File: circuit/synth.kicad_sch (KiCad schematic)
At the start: 3 parts, among them J1 Raspberry_Pi_4, U1 ADS1115IDGS

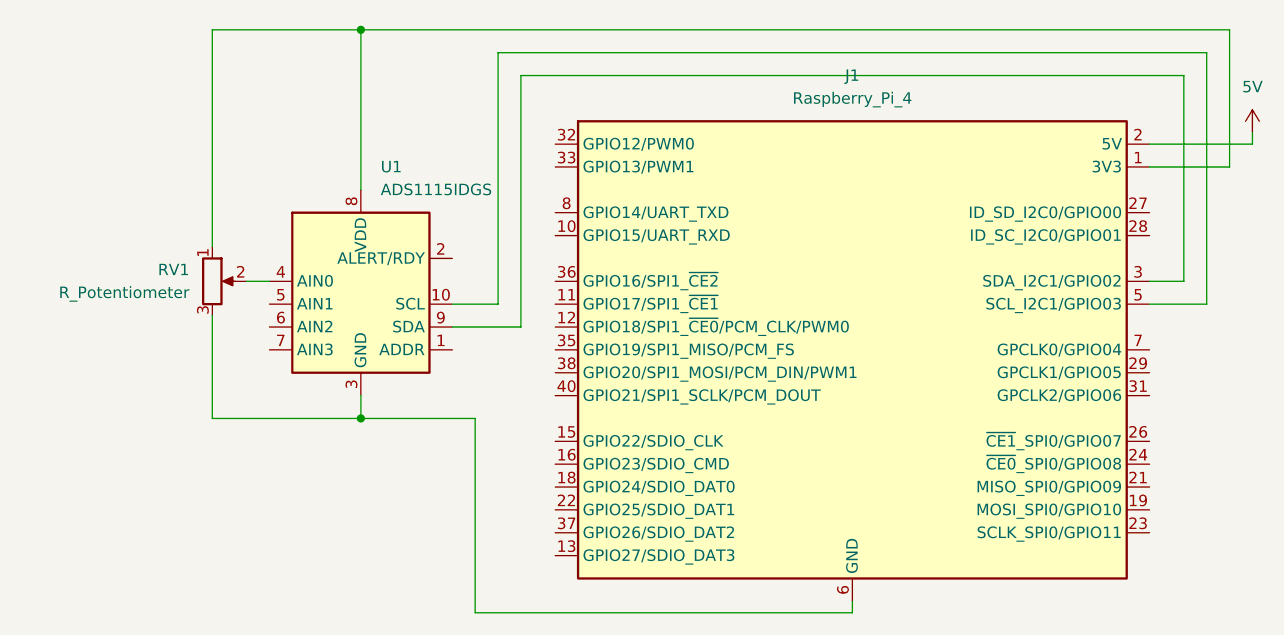
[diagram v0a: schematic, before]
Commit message: merge with Kicad file
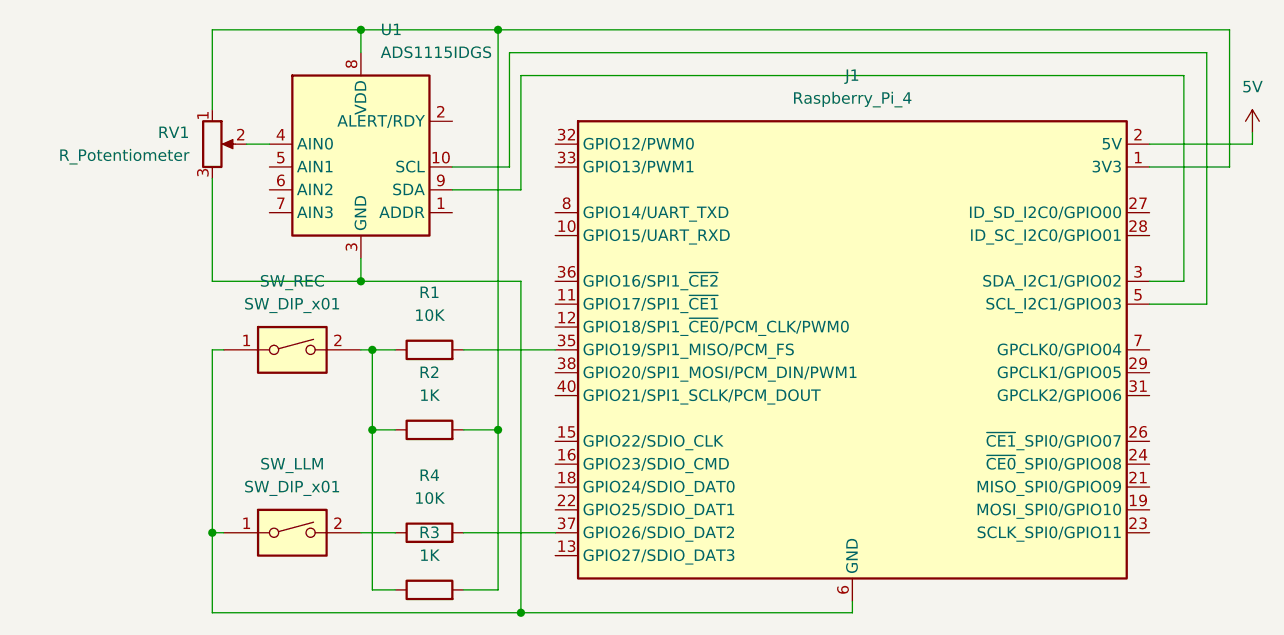
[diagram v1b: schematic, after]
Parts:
- added R1, R4: 10K, symbol Device:R
- added R2, R3: 1K, symbol Device:R
- added SW_LLM, SW_REC: SW_DIP_x01, symbol Switch:SW_DIP_x01
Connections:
- net at J1.1 (3V3), J1.17 (3V3), RV1.1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: now also R2.2, R3.2
- net at J1.14 (GND), J1.20 (GND), J1.25 (GND)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: now also SW_LLM.1, SW_REC.1
- net at J1.35 (GPIO19/SPI1_MISO/PCM_FS): now also R1.2
- net at J1.37 (GPIO26/SDIO_DAT2): now also R4.2
- new net: R1.1, R2.1, R3.1, SW_REC.2
- new net: R4.1, SW_LLM.2
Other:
- moved on the sheet: RV1, U1
